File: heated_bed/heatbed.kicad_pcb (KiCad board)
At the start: 2 copper layers, 8 parts, among them P1 CONN_POWER, P2 CONN_2

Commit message: Feita a primeira metade da PCB, com duas trilhas de aquecimento prontas. Restam as duas trilhas com menos interferencia externa
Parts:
- removed P2: CONN_2, 2PIN_6mm
- added MH1: MOUNTING_HOLE, MountingHole_3mm_RevA_Date21Jun2010, F.Cu at (36.0, 21.0)
- added MH2: MOUNTING_HOLE, MountingHole_3mm_RevA_Date21Jun2010, F.Cu at (245.0, 21.0)
- added MH3: MOUNTING_HOLE, MountingHole_3mm_RevA_Date21Jun2010, F.Cu at (245.0, 230.0)
- added MH4: MOUNTING_HOLE, MountingHole_3mm_RevA_Date21Jun2010, F.Cu at (36.0, 230.0)
- added PCB_R11: 4R, Track, B.Cu at (16.0, 40.0)
- added PCB_R21: 4R, Track, F.Cu at (89.1, 16.9)
- added PCB_R31, PCB_R41: 4R, Track, F.Cu at (248.1, 233.1)
- added TH1: 100k, SM0805, B.Cu at (140.5, 125.5)
- added TH2: 100k, SM0603, B.Cu at (142.5, 125.5)
- P1: value CONN_POWER -> CONN_4; footprint AK300-2 -> bornier4
- PCB_R1: footprint SM1206 -> Track1-1mm; moved to B.Cu
- PCB_R2, PCB_R3, PCB_R4: footprint SM1206 -> Track
- moved PCB_R2 250.4 mm to (86.5, 235.0), turned to 90 degrees
- moved PCB_R1 134.2 mm to (25.6, 131.7)
- moved P1 129.5 mm to (32.0, 125.5), turned to 270 degrees
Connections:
- D1 pad 1: N-000004 -> N-000001
- D1 pad 2: N-000001 -> N-0000010
- P1 pad 1: N-000005 -> N-000009
- P1 pad 2: N-000001 -> N-000003
- PCB_R1 pad 1: N-000001 -> N-0000010
- PCB_R2 pad 1: N-000001 -> N-0000010
- PCB_R2 pad 2: N-000005 -> N-000006
- PCB_R3 pad 1: N-000001 -> N-0000010
- PCB_R3 pad 2: N-000005 -> N-000007
- PCB_R4 pad 1: N-000001 -> N-0000010
- PCB_R4 pad 2: N-000005 -> N-000002
- R1 pad 1: N-000004 -> N-000009
- R1 pad 2: N-000005 -> N-000001
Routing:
- net N-000009: track 0.00 -> 12092.8 mm
- net N-0000010: track 0.00 -> 4238.5 mm
- net N-000003: track 0.00 -> 112.5 mm
- net N-000004: track 0.00 -> 112.2 mm
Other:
- board outline added: 220 x 215 mm
- net class Heating track added: clearance 0.2, trace_width 1.1, via_dia 0.889, via_drill 0.635
- net class Power distribution added: clearance 0.254, trace_width 4.5, via_dia 0.889, via_drill 0.635

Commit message: Roteadas as trilhas aquecidas, falta reposicionar furos
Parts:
- removed PCB_R1: 4R, Track1-1mm
- removed PCB_R11, PCB_R2, PCB_R21, PCB_R3, PCB_R31, PCB_R4, PCB_R41: 4R, Track
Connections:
- D1 pad 2: N-0000010 -> N-000005
- P1 pad 1: N-000009 -> N-000005
- P1 pad 4: N-0000010 -> N-000005
- R1 pad 1: N-000009 -> N-000005
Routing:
- net N-000005: track 0.00 -> 32225.9 mm
- net N-000009: track 12092.8 -> 0.00 mm
- net N-0000010: track 4238.5 -> 0.00 mm
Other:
- net class Heating track: clearance 0.2 -> 0.1524
- rule trace_min: 0.254 -> 0.1524
- rule via_min_size: 0.889 -> 0.1524

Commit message: Terminada a PCB, falta somente o silk.
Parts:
- D1, R1: moved to B.Cu
- moved D1 234.3 mm to (39.0, 231.0)
- moved R1 231.0 mm to (37.0, 228.0)
- moved MH1 4.00 mm to (32.0, 21.0)
- moved MH2 4.00 mm to (241.0, 21.0)
- moved MH3 4.00 mm to (241.0, 230.0)
- moved MH4 4.00 mm to (32.0, 230.0)
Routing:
- net N-000005: track 32225.9 -> 32299.5 mm
- net N-000003: track 0.00 -> 3.07 mm
- added copper zone on F.Cu, net (none)

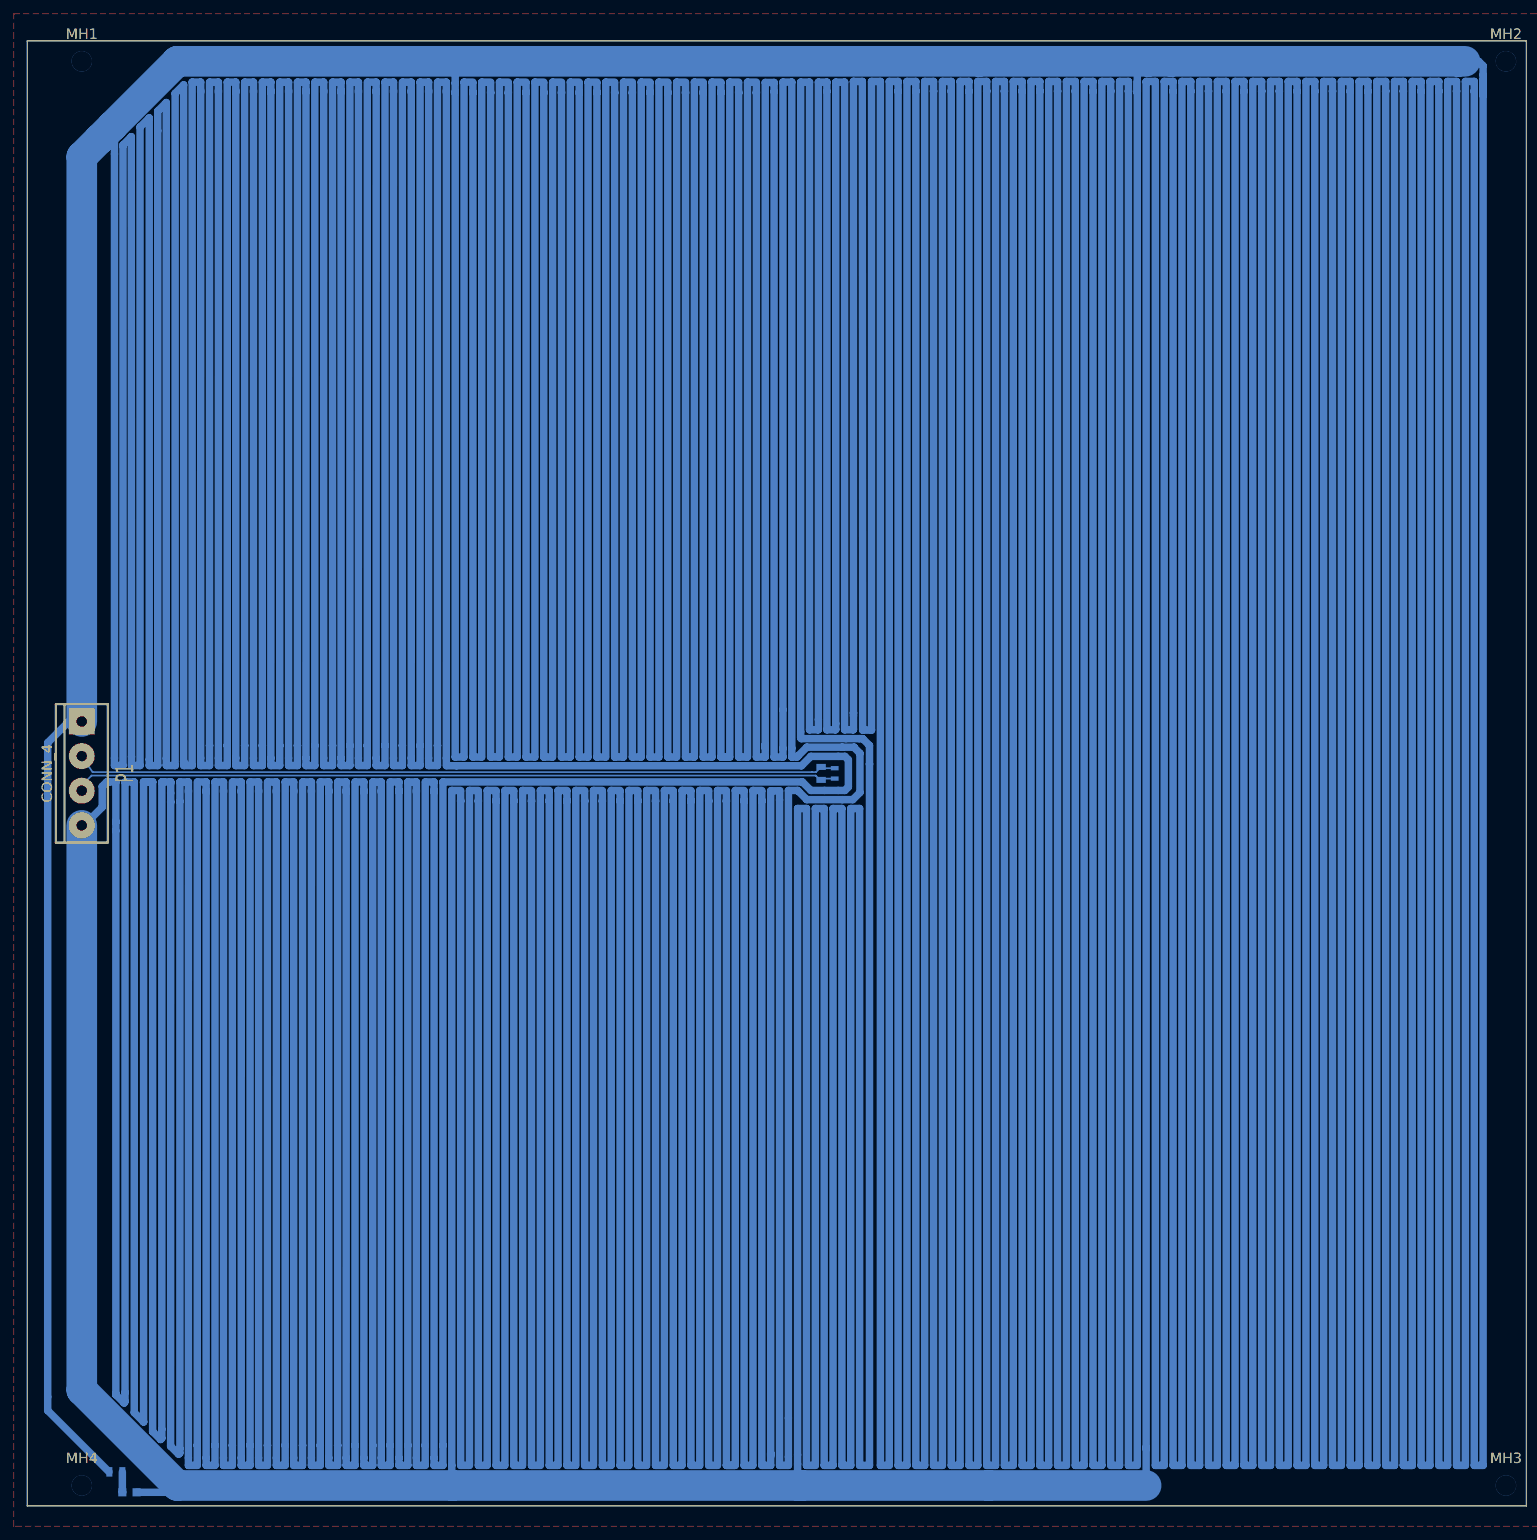
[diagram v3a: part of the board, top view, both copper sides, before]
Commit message: Placa finalizada
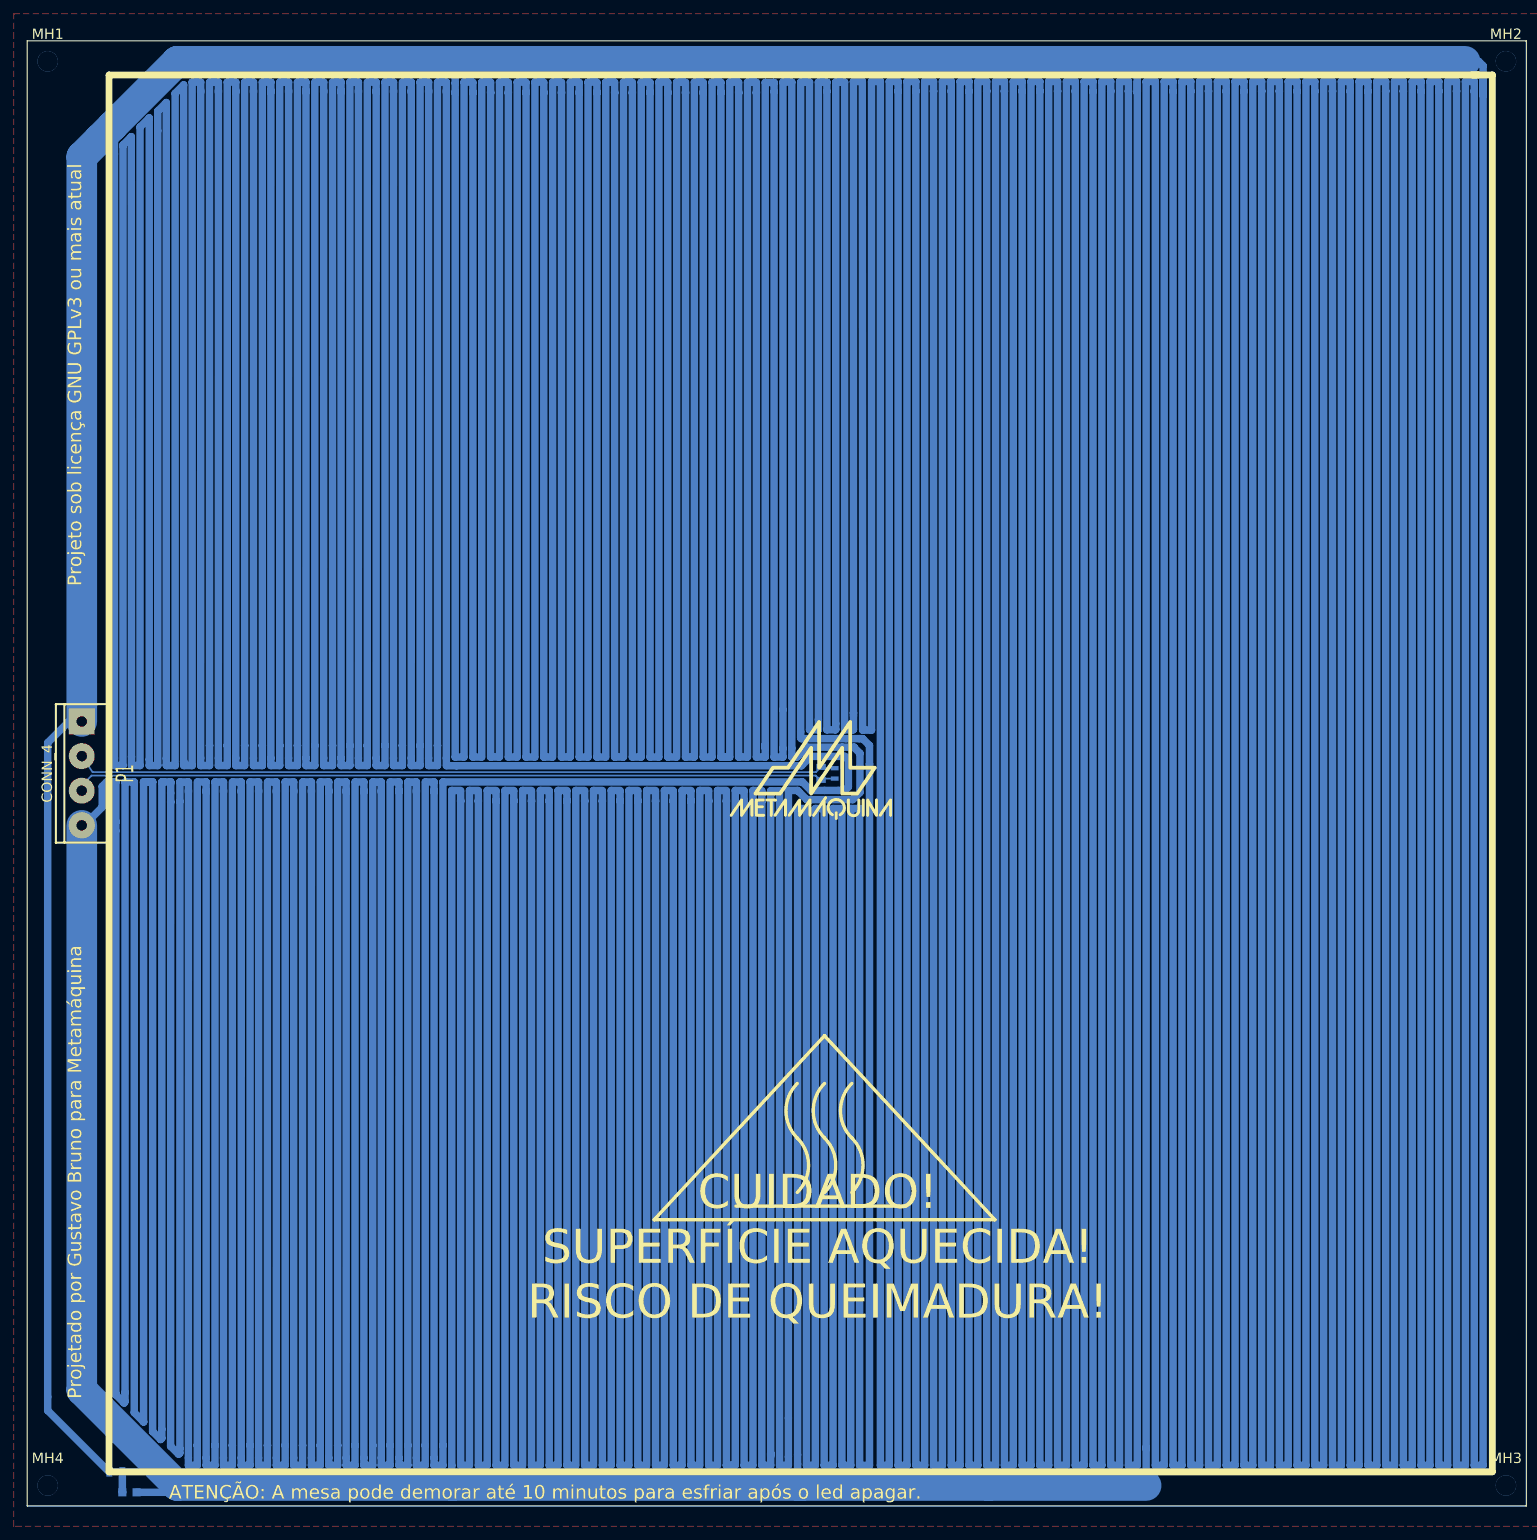
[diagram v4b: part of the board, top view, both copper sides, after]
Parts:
- added VAL: MM_logo, MM_logo, F.Cu at (139.0, 125.0)
- moved MH1 5.00 mm to (27.0, 21.0)
- moved MH4 5.00 mm to (27.0, 230.0)
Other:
- board text added: "ATENÇÃO: A mesa pode demorar até 10 minutos para esfriar após o led apagar."
- board text added: "CUIDADO! SUPERFÍCIE AQUECIDA! RISCO DE QUEIMADURA!"
- board text added: "Projetado por Gustavo Bruno para Metamáquina"
- board text added: "Projeto sob licença GNU GPLv3 ou mais atual"
